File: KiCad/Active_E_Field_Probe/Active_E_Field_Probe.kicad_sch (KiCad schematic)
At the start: 6 parts

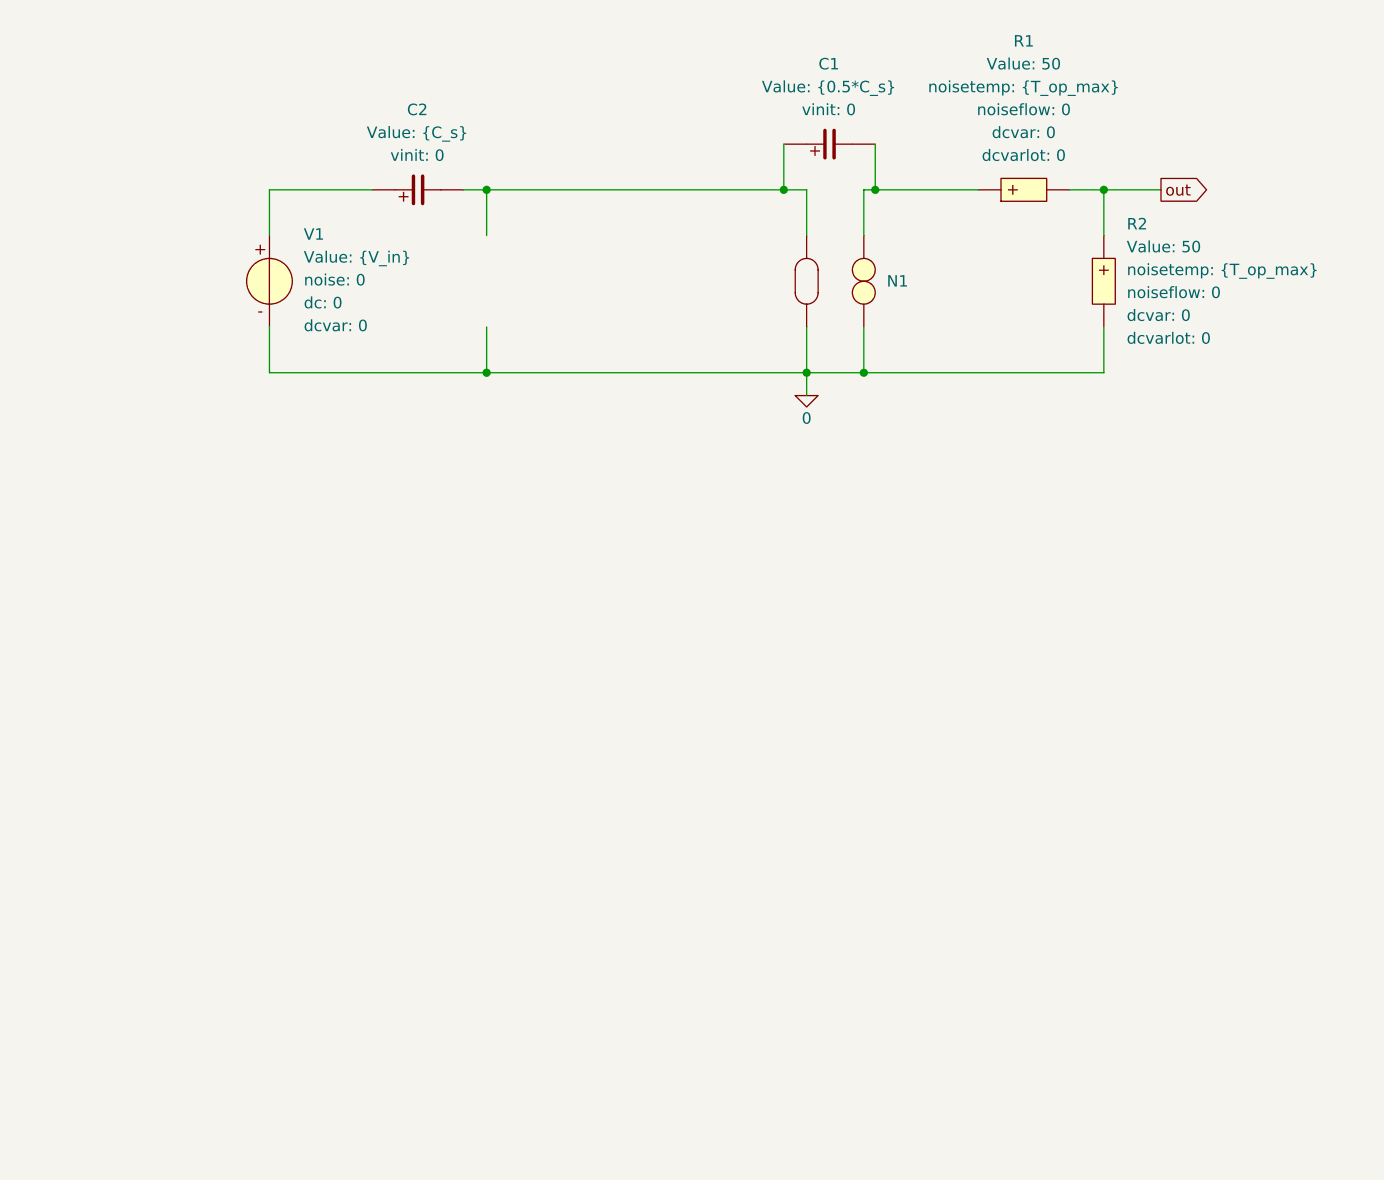
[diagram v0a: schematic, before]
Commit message: AAAAAAAAAAAHHHHH
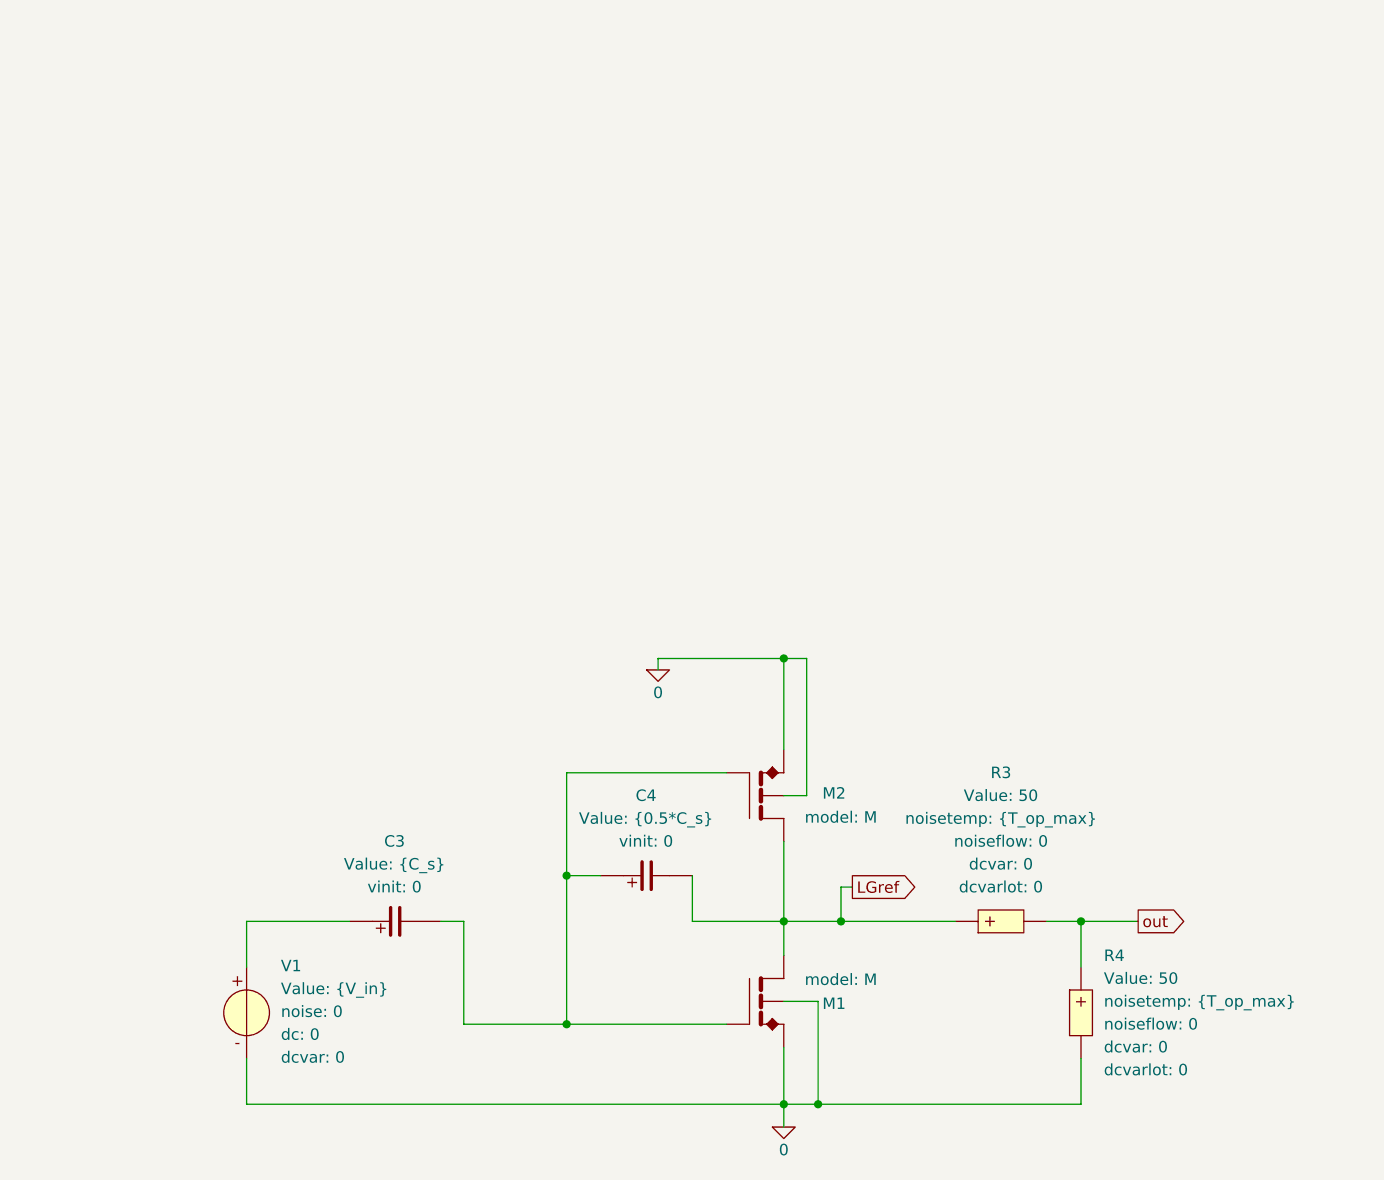
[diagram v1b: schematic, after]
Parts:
- removed C1: {0.5*C_s}, symbol SLiCAP:C
- removed C2: {C_s}, symbol SLiCAP:C
- removed N1: ~, symbol SLiCAP:N
- removed R1, R2: 50, symbol SLiCAP:R
- added C3: {C_s}, symbol SLiCAP:C
- added C4: {0.5*C_s}, symbol SLiCAP:C
- added M1, M2: ~, symbol SLiCAP:M
- added R3, R4: 50, symbol SLiCAP:R
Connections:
- net 0: now also M1.3 (S), M1.4 (B), M2.3 (S), M2.4 (B), R4.2
- net out: now also R3.2, R4.1
- net at V1.1 (p): now also C3.1
- new net: C3.2, C4.1, M1.2 (G), M2.2 (G)
- new net LGref: C4.2, M1.1 (D), M2.1 (D), R3.1

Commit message: 01-10 sesh
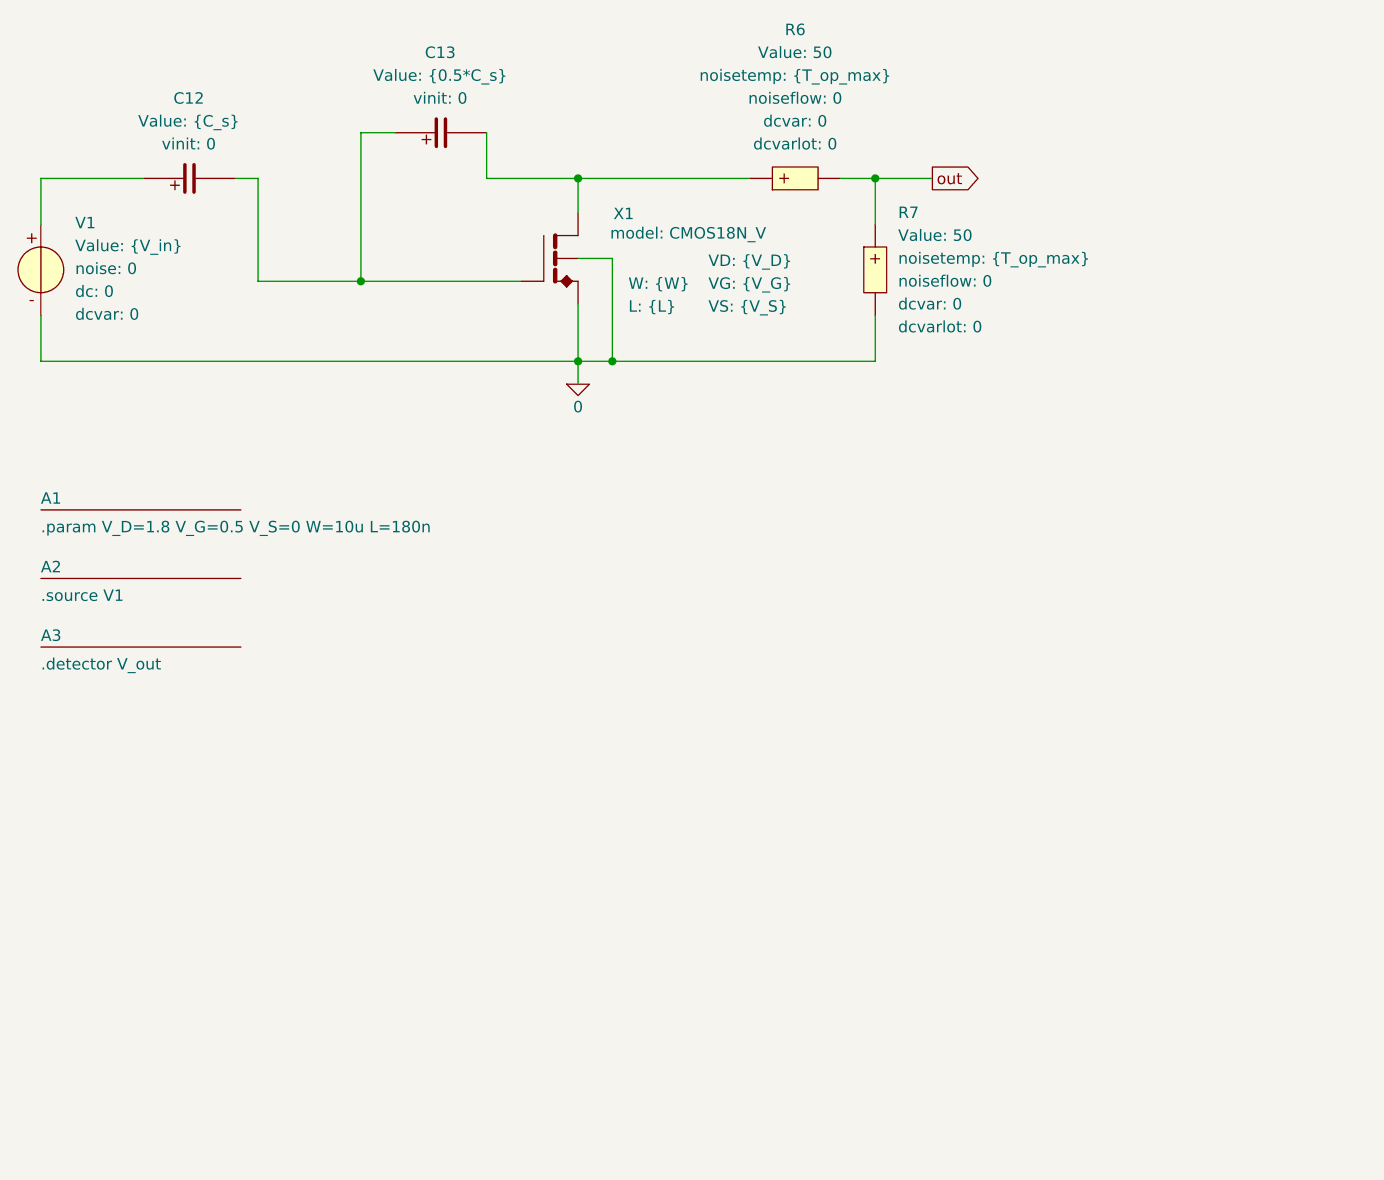
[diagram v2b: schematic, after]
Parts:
- removed C3: {C_s}, symbol SLiCAP:C
- removed C4: {0.5*C_s}, symbol SLiCAP:C
- removed M1, M2: ~, symbol SLiCAP:M
- removed R3, R4: 50, symbol SLiCAP:R
- added A1, A2, A3: ~, symbol SLiCAP:Command
- added C12: {C_s}, symbol SLiCAP:C
- added C13: {0.5*C_s}, symbol SLiCAP:C
- added R6, R7: 50, symbol SLiCAP:R
- added X1: ~, symbol SLiCAP:XMV
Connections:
- net 0: now also R7.2, X1.3 (S), X1.B (4)
- net out: now also R6.2, R7.1
- net at V1.1 (p): now also C12.1
- new net: C13.2, R6.1, X1.1 (D)
- new net: C12.2, C13.1, X1.2 (G)
